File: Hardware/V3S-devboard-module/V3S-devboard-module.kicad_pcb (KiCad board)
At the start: 4 copper layers, 31.9 x 52.9 mm, 84 parts, among them CN1 AS0BC21-S30BE-7H, J201 Micro_SD_Card_Det1, J301 AS0BC21-S30BE-7H, U101 EA3036C, U102 XC6206PxxxMR, U201 V3S, U202 W25Q128JVS, Y201 Crystal_Small, Y202 Crystal_GND24_Small

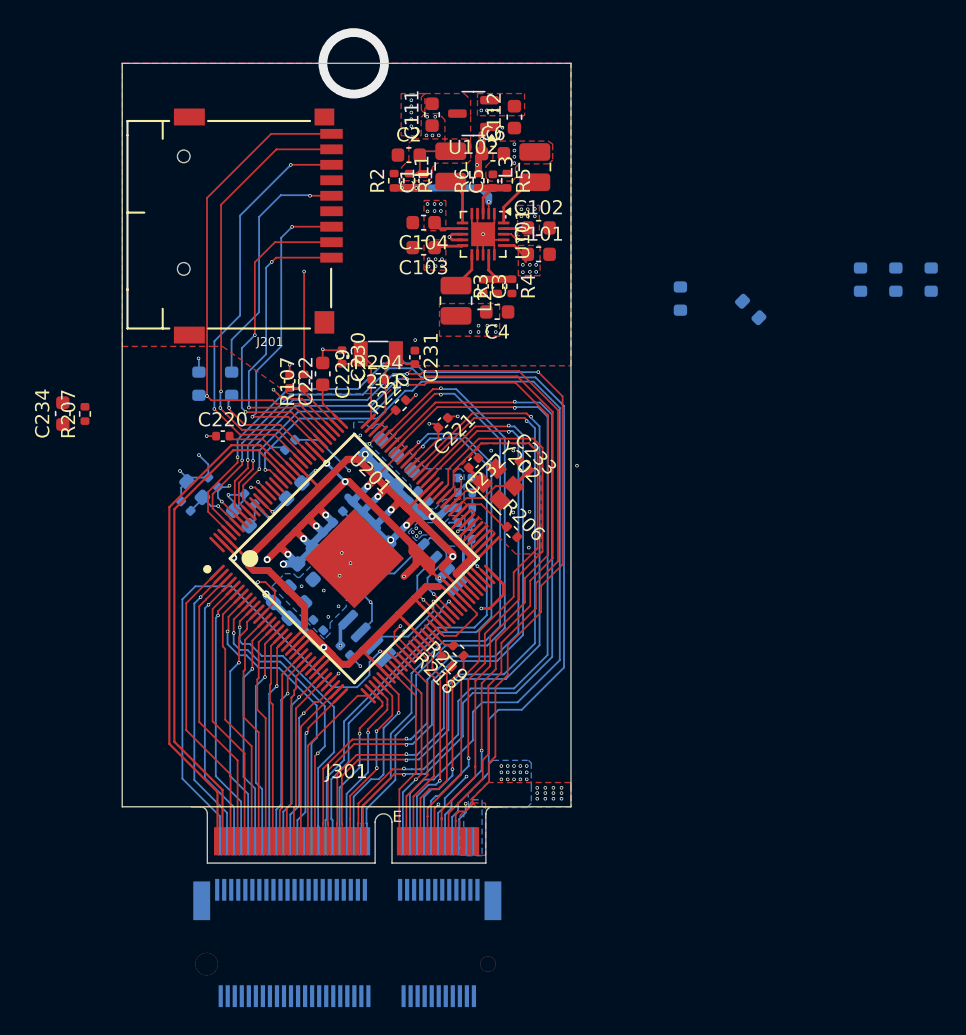
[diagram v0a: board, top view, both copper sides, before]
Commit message: layout
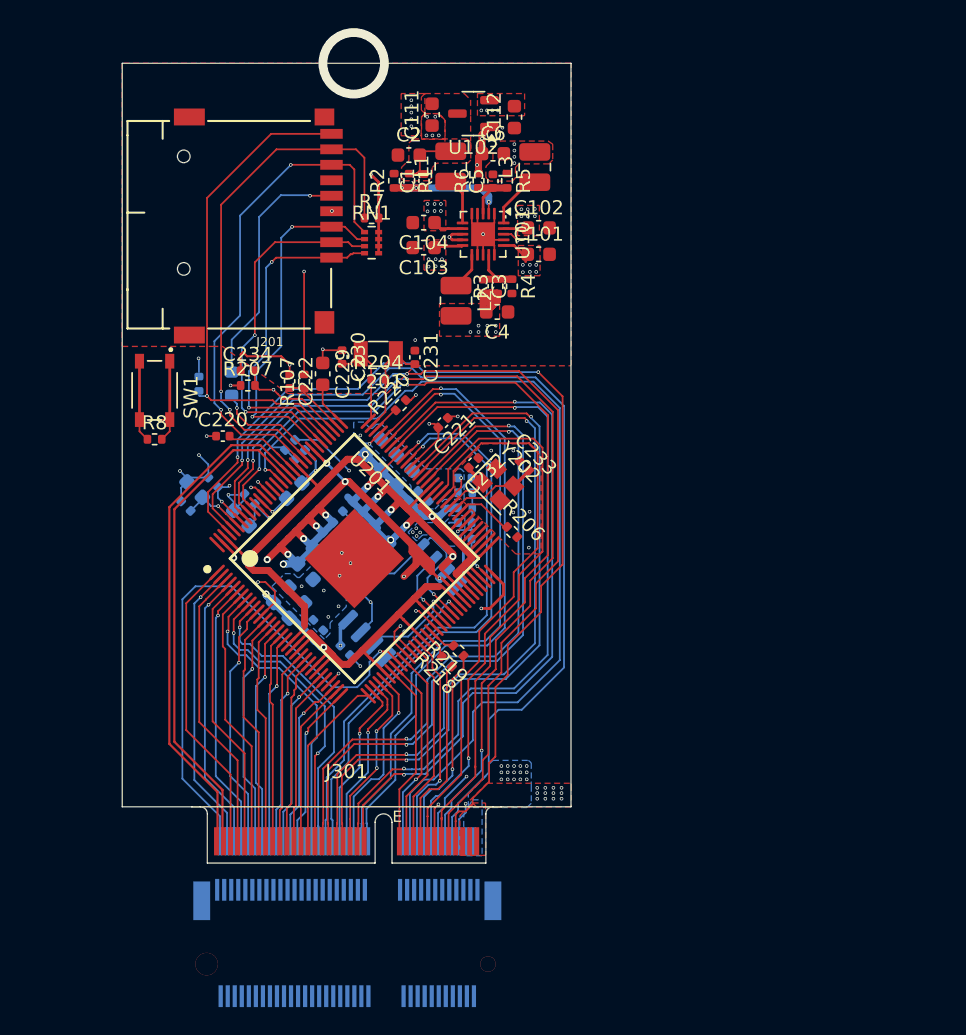
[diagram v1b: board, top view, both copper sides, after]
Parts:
- removed R211, R212, R213, R214, R215: 10k, Resistor_SMD:R_0603_1608Metric
- added C7: 1n, Capacitor_SMD:C_0402_1005Metric, B.Cu at (148.4, 90.5)
- added R7: 10k, Resistor_SMD:R_0402_1005Metric, F.Cu at (153.5, 73.7)
- added R8: 0, Resistor_SMD:R_0402_1005Metric, F.Cu at (138.1, 89.5)
- added RN1: R_Pack04, Resistor_SMD:R_Array_Concave_4x0402, F.Cu at (153.5, 75.5)
- added SW1: SW_MEC_5E, v3s-devboard-module:SW_SKRPACE010, F.Cu at (138.1, 86.0)
- C234: value 1u -> 100n; footprint Capacitor_SMD:C_0603_1608Metric -> Capacitor_SMD:C_0402_1005Metric
- R210: footprint Resistor_SMD:R_0603_1608Metric -> Resistor_SMD:R_0402_1005Metric
- moved C234 13.5 mm to (144.7, 84.6), turned to 0 degrees
- moved R207 11.7 mm to (144.7, 85.6), turned to 0 degrees
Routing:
- net SPI.MISO: track 5.46 -> 49.9 mm, vias 1 -> 2
- net GND: track 41.3 -> 54.0 mm, vias 54 -> 53
- net 3V3: track 166.2 -> 174.3 mm, vias 26 -> 30
- net SDC0.D0: track 31.4 -> 38.1 mm
- net SDC0.D1: track 30.2 -> 36.6 mm
- net 1V8: track 56.0 -> 61.8 mm
- net SDC0.CMD: track 22.9 -> 25.7 mm
- net RESET: track 57.3 -> 59.8 mm
- net SDC0.D2: track 21.7 -> 24.1 mm
- net SDC0.D3: track 23.3 -> 25.8 mm
- net LRADC0: track 64.6 -> 65.7 mm
